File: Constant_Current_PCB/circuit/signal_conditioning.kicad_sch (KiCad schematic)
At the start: 7 parts, among them J2 Screw_Terminal_01x03, J3 Screw_Terminal_01x02, Q1 NPN, U3 TL081CP

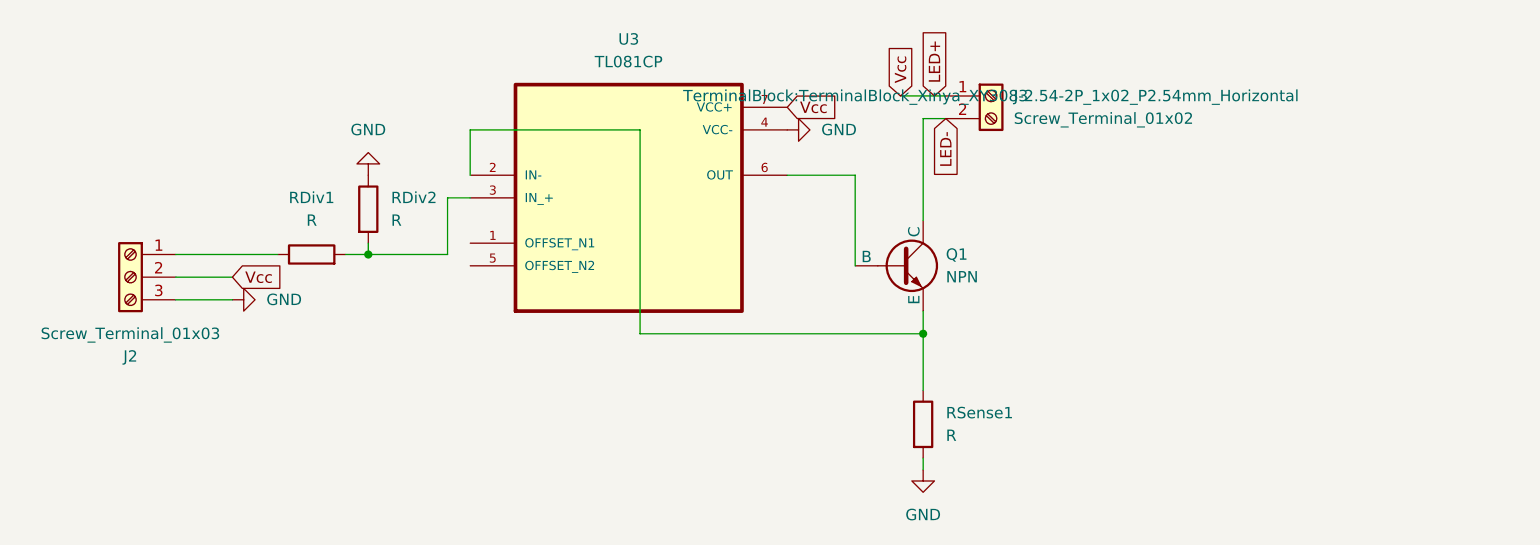
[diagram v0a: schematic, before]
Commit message: component list
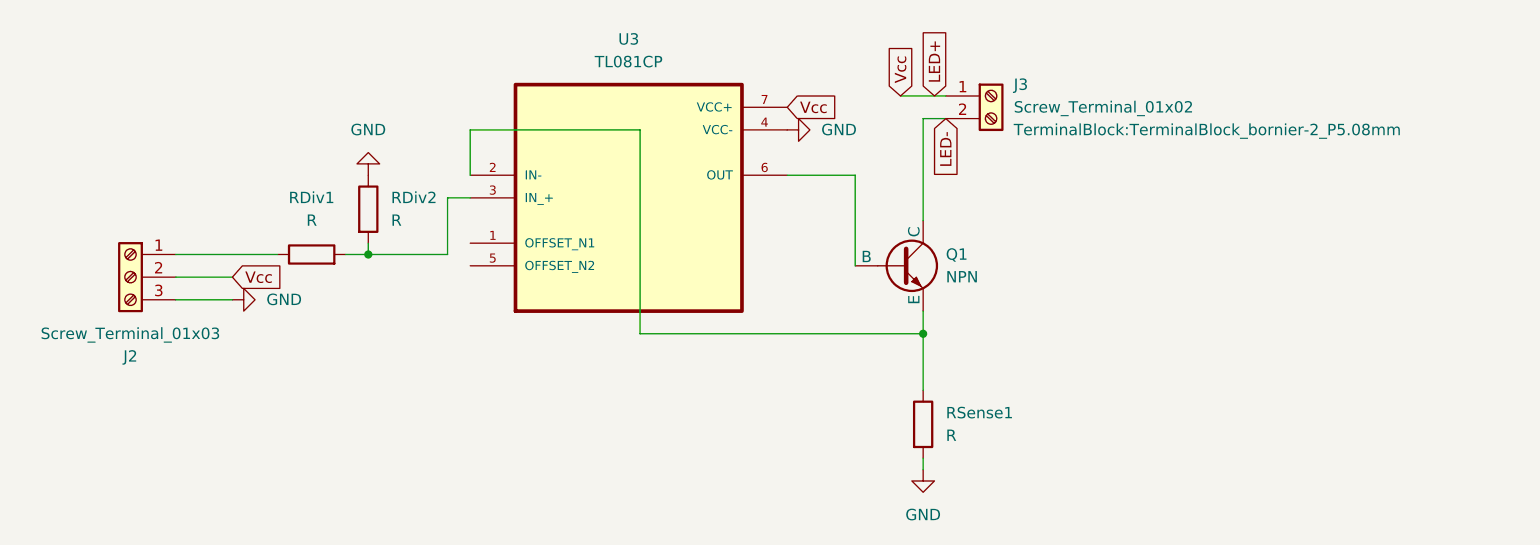
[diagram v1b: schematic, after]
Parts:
- J2: footprint TerminalBlock:TerminalBlock_Xinya_XY308-2.54-3P_1x03_P2.54mm_Horizontal -> TerminalBlock:TerminalBlock_bornier-3_P5.08mm
- J3: footprint TerminalBlock:TerminalBlock_Xinya_XY308-2.54-2P_1x02_P2.54mm_Horizontal -> TerminalBlock:TerminalBlock_bornier-2_P5.08mm
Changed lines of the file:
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@@
 			)
 		)
-		(property "Footprint" "TerminalBlock:TerminalBlock_Xinya_XY308-2.54-3P_1x03_P2.54mm_Horizontal"
+		(property "Footprint" "TerminalBlock:TerminalBlock_bornier-3_P5.08mm"
 			(at 78.74 85.09 0)
 			(effects
@@
 		(fields_autoplaced yes)
 		(property "Reference" "J3"
-			(at 177.8 64.7699 0)
+			(at 177.8 63.4999 0)
 			(effects
 				(font
@@
 		)
 		(property "Value" "Screw_Terminal_01x02"
-			(at 177.8 67.3099 0)
+			(at 177.8 66.0399 0)
 			(effects
 				(font
@@
 			)
 		)
-		(property "Footprint" "TerminalBlock:TerminalBlock_Xinya_XY308-2.54-2P_1x02_P2.54mm_Horizontal"
-			(at 175.26 64.77 0)
+		(property "Footprint" "TerminalBlock:TerminalBlock_bornier-2_P5.08mm"
+			(at 177.8 68.5799 0)
 			(effects
 				(font
 					(size 1.27 1.27)
 				)
+				(justify left)
 			)
 		)
